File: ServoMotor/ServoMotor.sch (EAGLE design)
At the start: 30 parts, among them Q1 TIP120, Q2 TIP120, Y1 16MHz

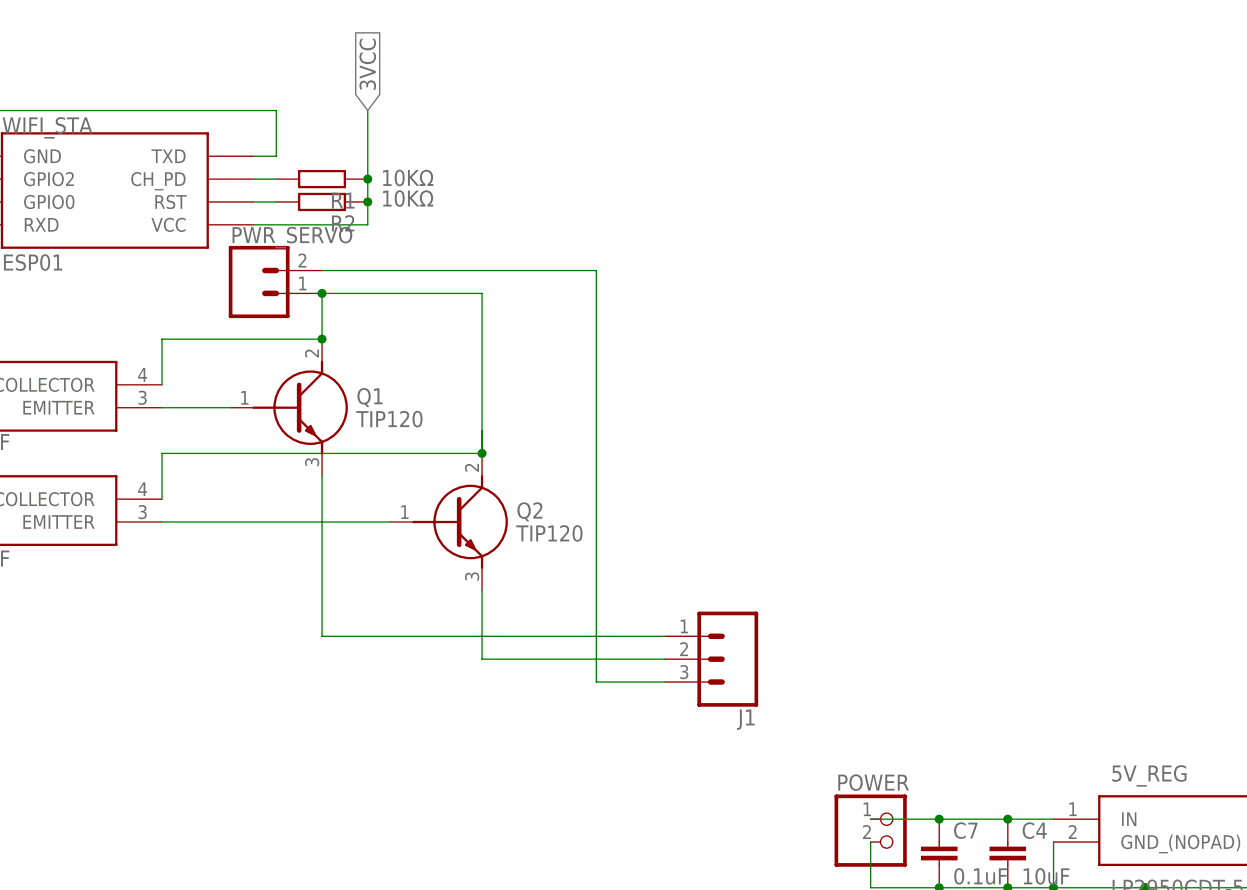
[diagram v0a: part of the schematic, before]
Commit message: Updated ServoMotor
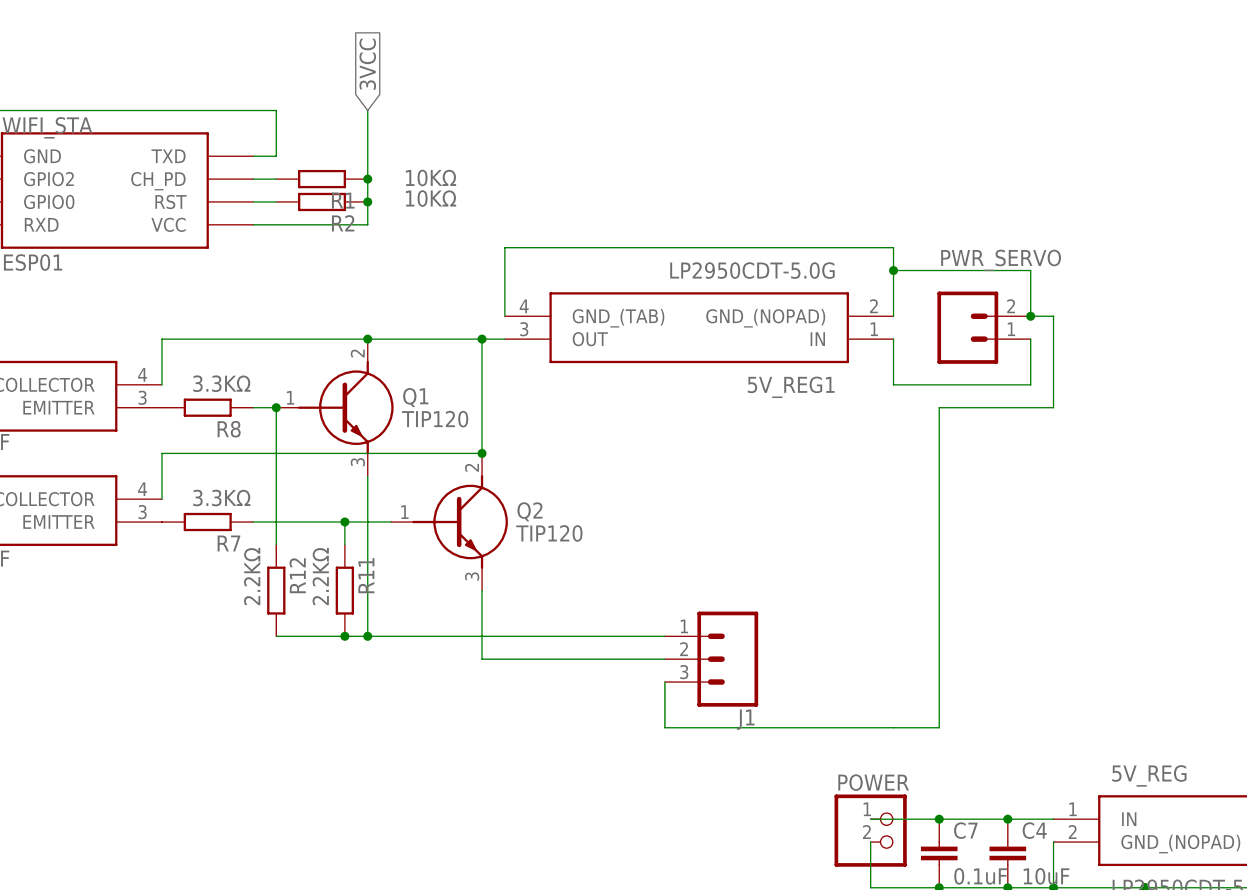
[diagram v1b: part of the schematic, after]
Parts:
- added 5V_REG1: LP2950CDT-5.0G, LP2950CDT-5.0G:LP2950CDT-5.0G
- added R11, R12: 2.2KΩ, eagle-ltspice:RR1210
- added R7, R8: 3.3KΩ, eagle-ltspice:RR1210
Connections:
- new net N$5: OPTO1.EMITTER, R7.2
- new net N$7: Q2.B, R11.1, R7.1
- new net N$8: 5V_REG1.IN, PWR_SERVO.1
- net N$2: now also R8.2; no longer Q1.B
- net N$3: now also Q1.B, R12.1, R8.1; no longer OPTO1.EMITTER, Q2.B
- net PWR_SERVO_VCC: now also 5V_REG1.OUT; no longer PWR_SERVO.1
- net SERVO_GND: now also 5V_REG1.GND_(NOPAD), 5V_REG1.GND_(TAB)
- net SERVO_VCC: now also R11.2, R12.2
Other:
- moved on the sheet: PWR_SERVO, Q1
